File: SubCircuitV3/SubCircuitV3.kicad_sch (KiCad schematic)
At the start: 48 parts, among them J1 JTAG, J10 ESC_POWER, J11 ESC_POWER, J12 ESC_POWER, J13 ESC_POWER, J14 FEMALE XT-60, J15 ESC PWM, J16 5S, J17 Water Sensor Input, J18 3S OUT, J19 2S OUT, J2 ESC PWM, J20 SWITCH, J3 ESC PWM, J4 ESC PWM, J5 ESC PWM, J6 ESC PWM, J7 3S, J8 ESC_POWER, J9 ESC_POWER, K1 G5Q-1A, Q1 NMOS, Q2 NMOS, Q3 NMOS, Q4 NMOS, Q5 NMOS, Q6 NMOS

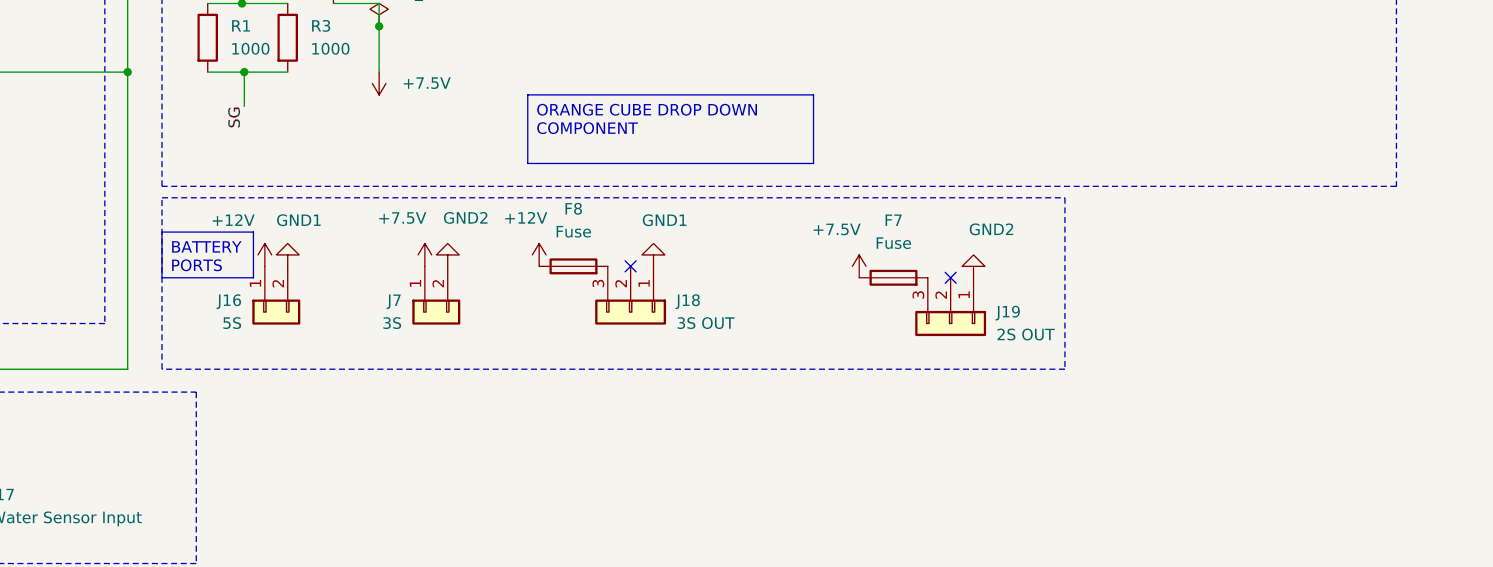
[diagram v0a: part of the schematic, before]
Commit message: Version 4
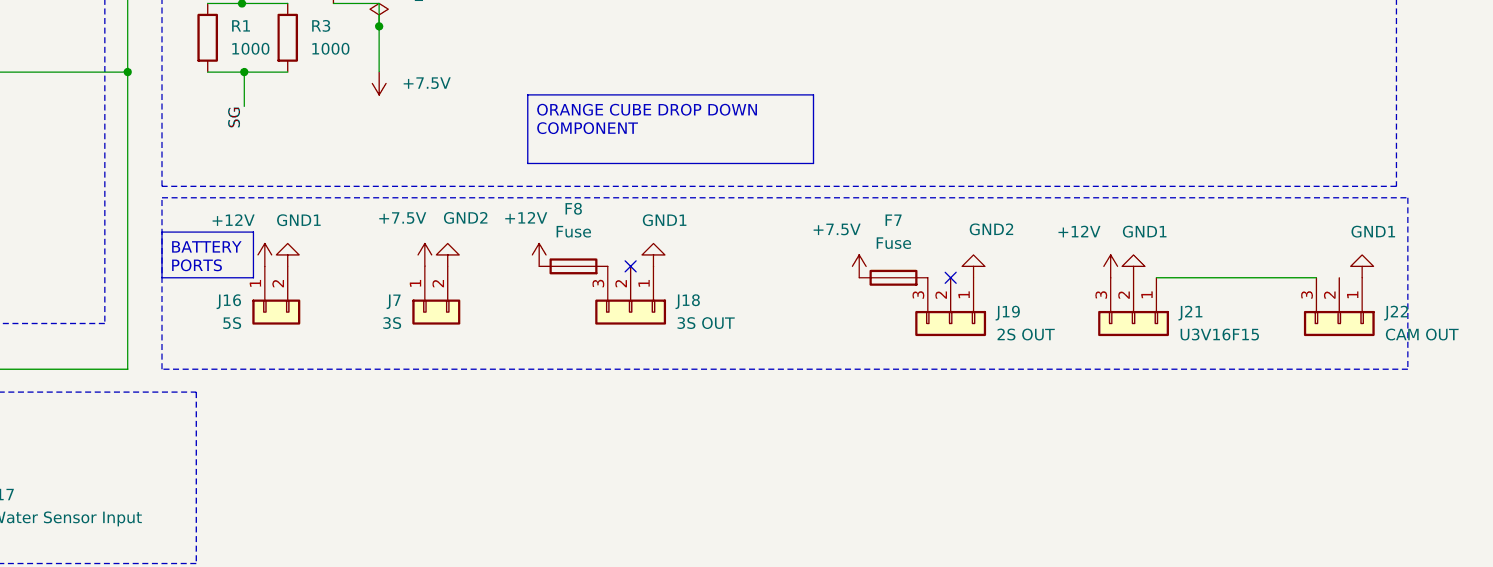
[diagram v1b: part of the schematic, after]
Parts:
- added J21: U3V16F15, Connector_PinHeader_2.54mm:PinHeader_1x03_P2.54mm_Vertical, symbol Connector_Generic:Conn_01x03
- added J22: CAM OUT, 284932-3:CONN3_284392-3_TEC, symbol Connector_Generic:Conn_01x03
- C1, C2: footprint Capacitor_WCAP-ATG8_5x11_WRE:CAP_WCAP-ATG8_5x11_WRE -> Capacitor_THT:C_Radial_D8.0mm_H7.0mm_P3.50mm
- F7: footprint Resistor_THT:R_Axial_DIN0411_L9.9mm_D3.6mm_P20.32mm_Horizontal -> Resistor_THT:R_Axial_Power_L25.0mm_W9.0mm_P30.48mm
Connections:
- net +12V: now also J21.3 (Pin_3)
- net GND1: now also J21.2 (Pin_2), J22.1 (Pin_1)
- new net: J21.1 (Pin_1), J22.3 (Pin_3)
